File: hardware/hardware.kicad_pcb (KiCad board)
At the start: 2 copper layers, 141.7 x 73.6 mm, 78 parts, among them J1 USB_C_Receptacle_USB2.0, J2 AudioPlug4, J3 USB_C_Receptacle_USB2.0, J4 AudioPlug4, SW1 SW_Push, SW2 SW_Push, SW3 SW_Push, SW4 SW_Push, SW5 SW_Push, SW6 SW_Push, SW7 SW_Push, SW8 SW_Push, SW9 SW_Push, U3 ATMEGA32U4, Y1 16MHz

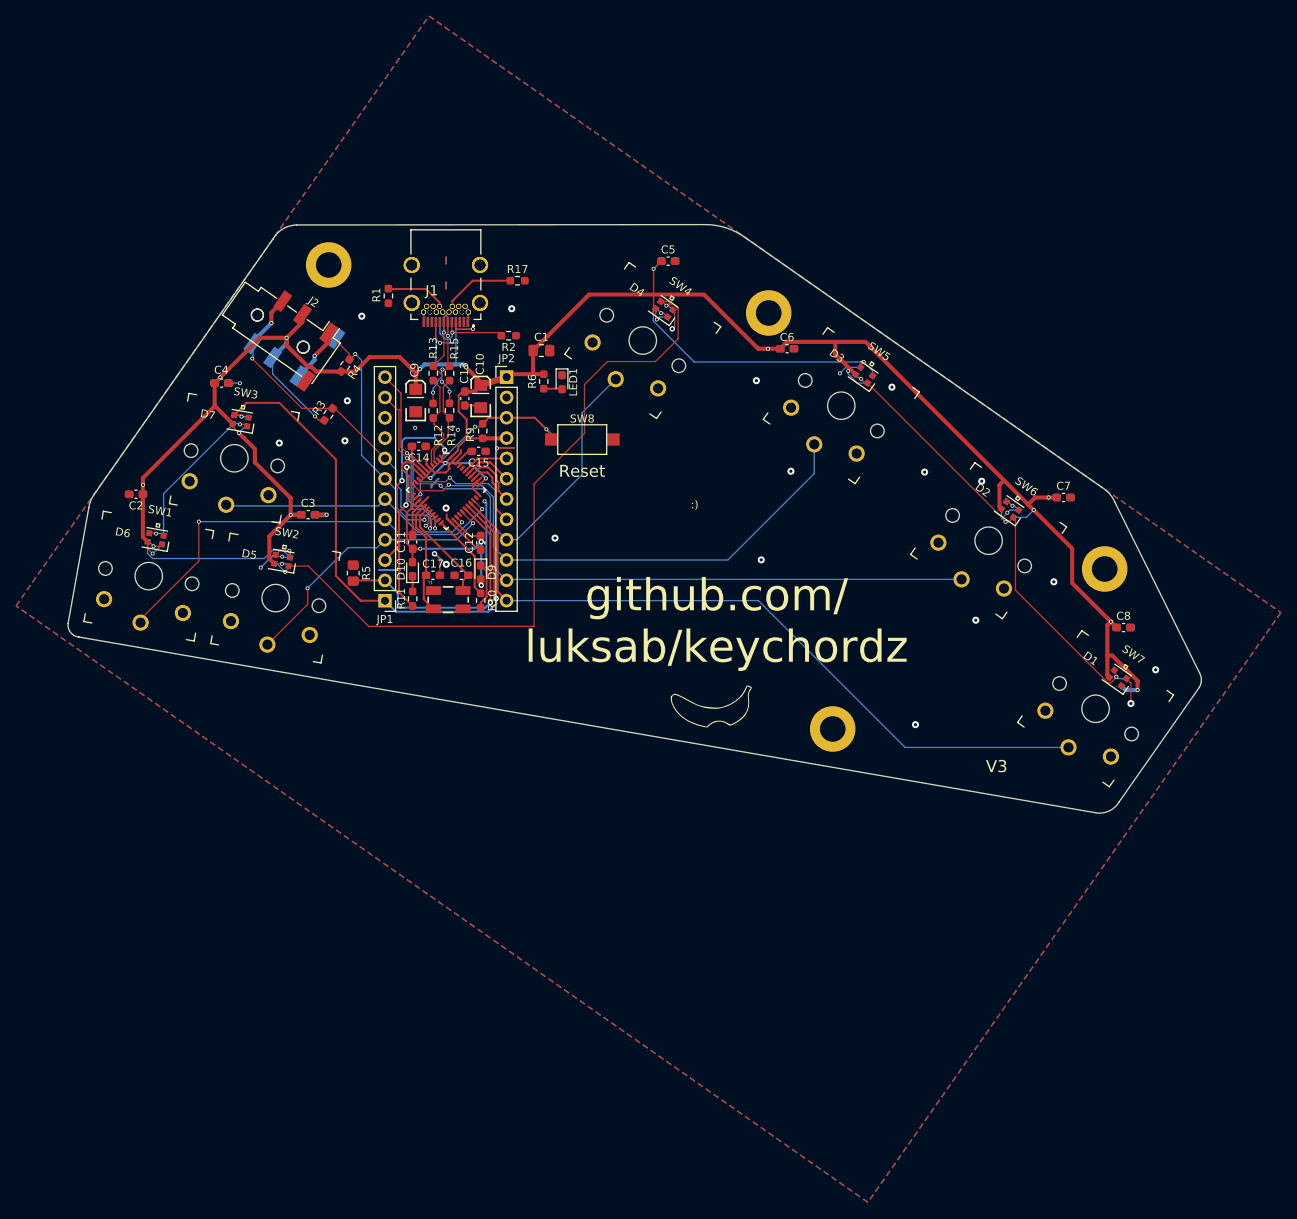
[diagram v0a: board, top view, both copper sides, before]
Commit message: oder V3
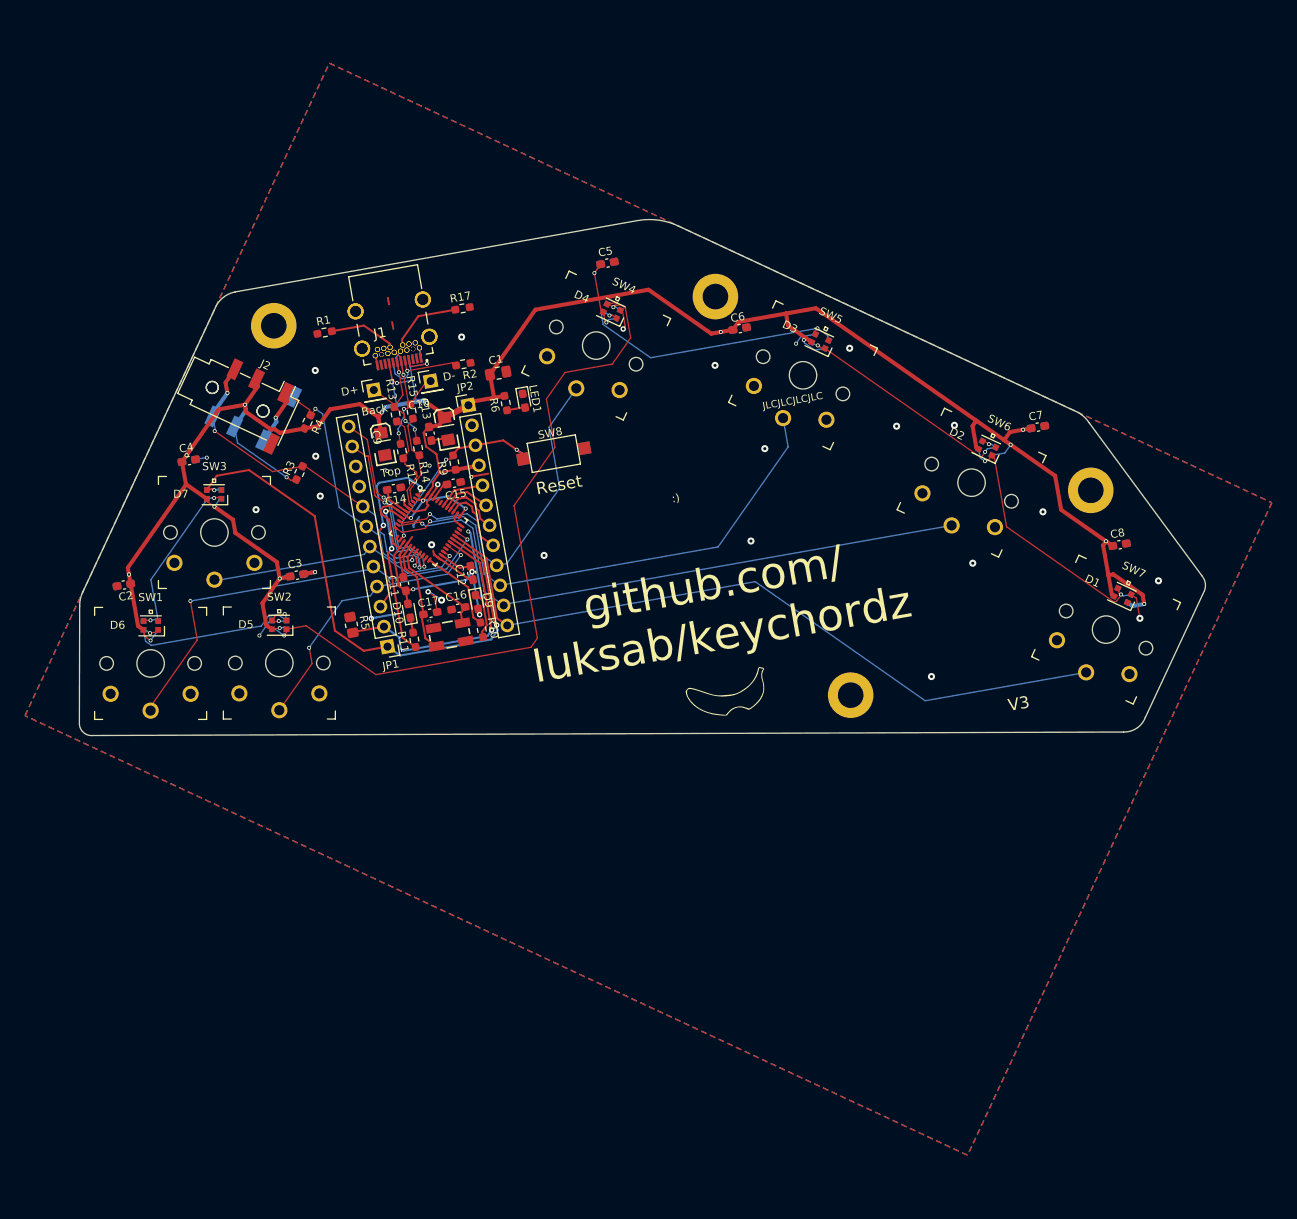
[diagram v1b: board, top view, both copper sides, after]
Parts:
- added D+: PinHeader_1x01_P2.54mm_Vertical, Connector_PinHeader_2.54mm:PinHeader_1x01_P2.54mm_Vertical, F.Cu at (30.6, 17.6)
- added D-: PinHeader_1x01_P2.54mm_Vertical, Connector_PinHeader_2.54mm:PinHeader_1x01_P2.54mm_Vertical, F.Cu at (37.7, 16.5)
- moved C2 11.4 mm to (-0.61, 42.0), turned to -170 degrees
- moved C23 11.4 mm to (-0.61, 42.0), turned to -170 degrees
- moved SW1 10.9 mm to (2.74, 51.8), turned to 0 degrees
- moved D15 10.8 mm to (2.77, 47.1), turned to 180 degrees
- moved D6 10.8 mm to (2.77, 47.1), turned to 0 degrees
- moved C24 10.5 mm to (7.51, 26.5), turned to 10 degrees
- moved C4 10.5 mm to (7.51, 26.5), turned to 10 degrees
- moved C19 10.4 mm to (123.9, 37.0), turned to 10 degrees
- moved C8 10.4 mm to (123.9, 37.0), turned to 10 degrees
- moved D1 10.3 mm to (124.2, 43.3), turned to -25 degrees
- moved D8 10.3 mm to (124.2, 43.3), turned to 155 degrees
- moved REF** 10.2 mm to (18.1, 9.59), turned to 10 degrees
- moved SW7 9.98 mm to (122.2, 47.6), turned to -25 degrees
- moved REF** 9.98 mm to (120.3, 30.2), turned to 10 degrees
- moved J2 9.83 mm to (14.8, 19.3), turned to -25 degrees
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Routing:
- net Net-(R15-Pad1): track 14.6 -> 18.6 mm
- net Net-(J3-PadA6): track 14.4 -> 17.8 mm
- net Net-(J1-PadB5): track 7.61 -> 8.38 mm
- net Net-(D4-Pad4): track 92.4 -> 91.8 mm
- net GND: track 66.1 -> 66.2 mm, vias 29 -> 31
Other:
- board size 141.7 x 73.6 mm -> 140.8 x 64.5 mm
- board text added: "Back"
- board text added: "JLCJLCJLCJLC"
- board text added: "Top"
